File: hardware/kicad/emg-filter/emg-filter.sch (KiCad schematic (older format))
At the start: 0 parts

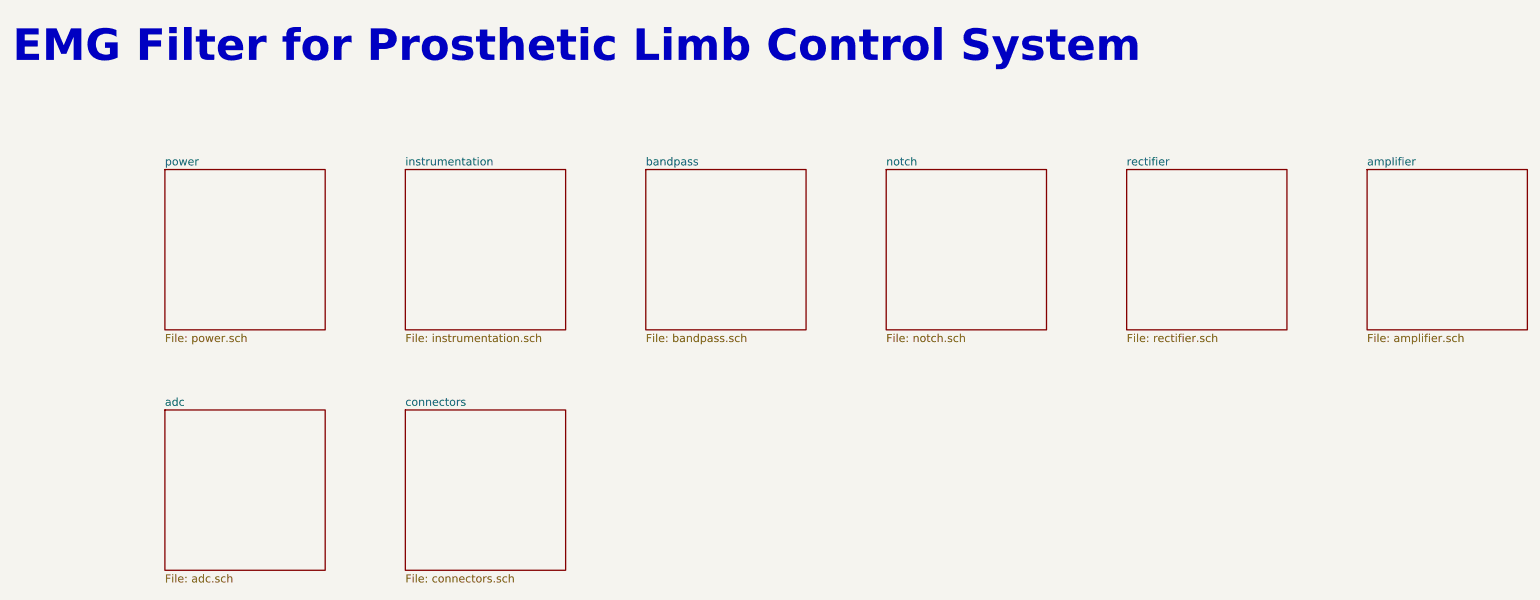
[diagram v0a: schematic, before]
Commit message: minor fixes
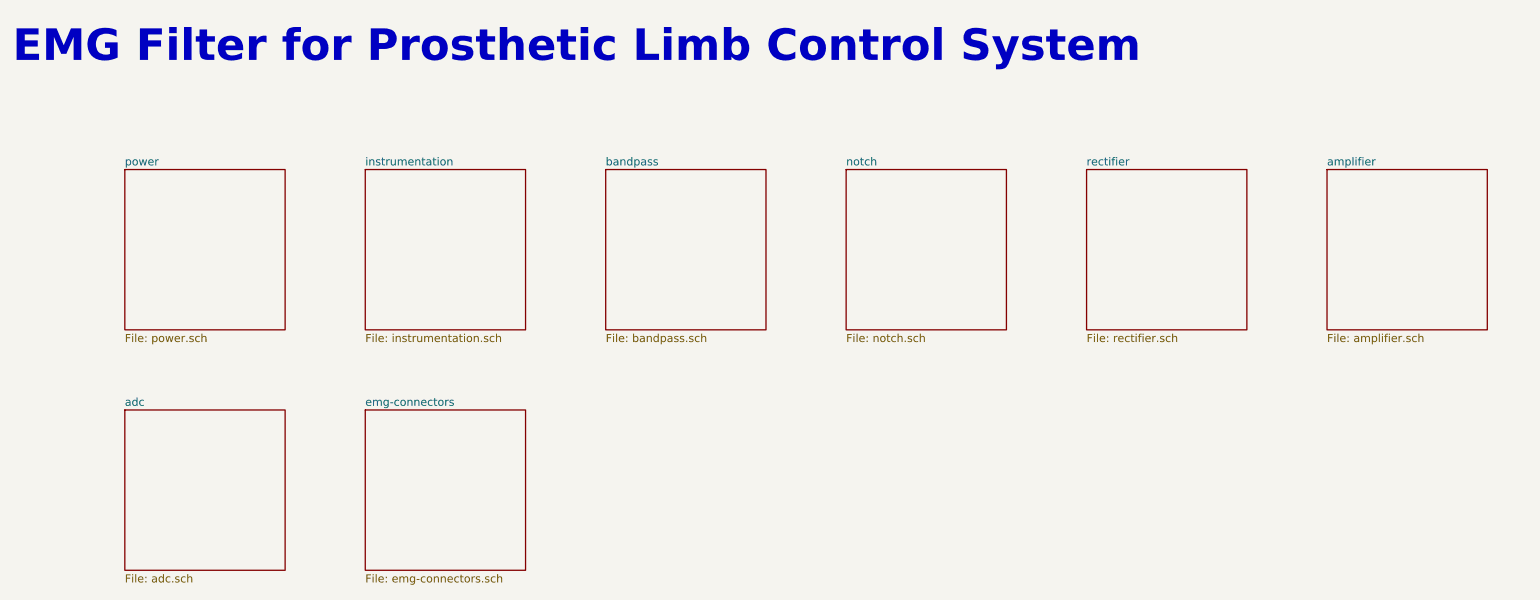
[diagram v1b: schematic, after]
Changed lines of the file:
@@
 $EndDescr
 $Sheet
-S 1500 1500 1000 1000
+S 1250 1500 1000 1000
 U 61C38667
 F0 "power" 50
@@
 $EndSheet
 $Sheet
-S 3000 1500 1000 1000
+S 2750 1500 1000 1000
 U 61C386B1
 F0 "instrumentation" 50
@@
 $EndSheet
 $Sheet
-S 4500 1500 1000 1000
+S 4250 1500 1000 1000
 U 61C386E2
 F0 "bandpass" 50
@@
 $EndSheet
 $Sheet
-S 6000 1500 1000 1000
+S 5750 1500 1000 1000
 U 61C38708
 F0 "notch" 50
@@
 $EndSheet
 $Sheet
-S 7500 1500 1000 1000
+S 7250 1500 1000 1000
 U 61C38746
 F0 "rectifier" 50
@@
 $EndSheet
 $Sheet
-S 9000 1500 1000 1000
+S 8750 1500 1000 1000
 U 61C38776
 F0 "amplifier" 50
@@
 $EndSheet
 $Sheet
-S 1500 3000 1000 1000
+S 1250 3000 1000 1000
 U 61C38939
 F0 "adc" 50
@@
 $EndSheet
 $Sheet
-S 3000 3000 1000 1000
+S 2750 3000 1000 1000
 U 61C389A8
-F0 "connectors" 50
-F1 "connectors.sch" 50
+F0 "emg-connectors" 50
+F1 "emg-connectors.sch" 50
 $EndSheet
 Text Notes 550  850  0    197  ~ 39
